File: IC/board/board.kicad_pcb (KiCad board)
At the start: 4 copper layers, 72.6 x 51.6 mm, 36 parts, among them Q1 IRLZ44N, SW1 SW_Push, SW2 SW_Push, SW3 SW_Push, SW4 SW_Push, SW5 SW_Push, SW6 Rotary_Encoder_Switch, U1 L7805, U2 ATmega328P-PU, Y1 16Mhz

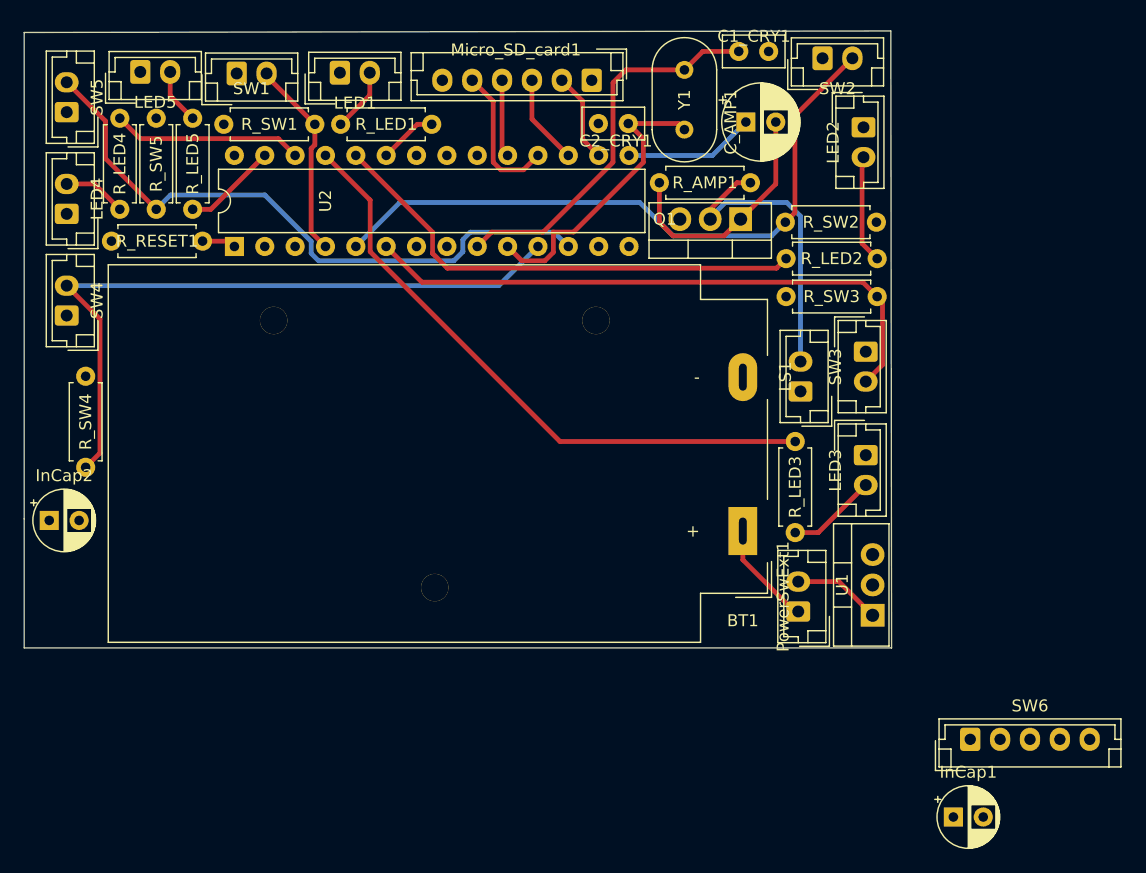
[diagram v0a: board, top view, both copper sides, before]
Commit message: Update to las kicad version
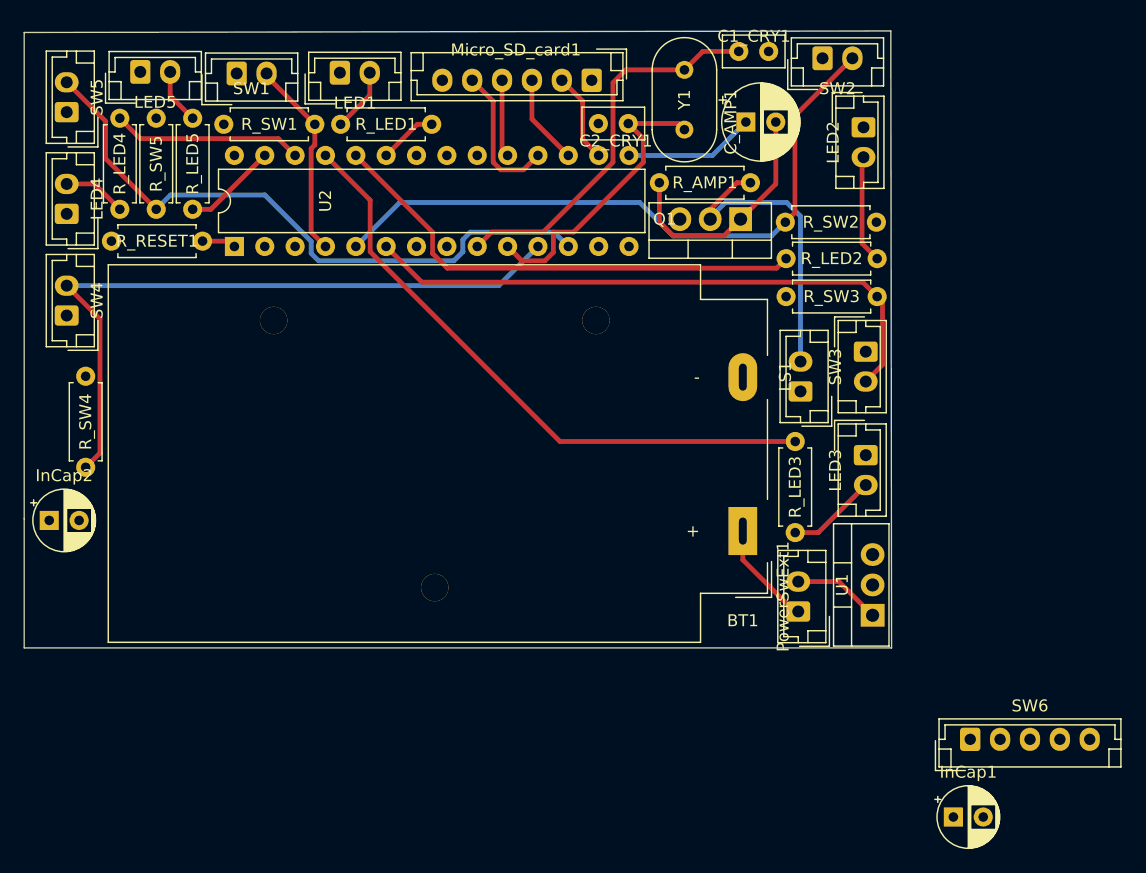
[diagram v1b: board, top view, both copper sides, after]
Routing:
- added copper zone on In1.Cu, net Net-(BT1-Pad2)
- added copper zone on In2.Cu, net Net-(InCap2-Pad1)
- removed copper zone on Ground, net Net-(BT1-Pad2)
- removed copper zone on Power, net Net-(InCap2-Pad1)
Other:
- net class Default removed
